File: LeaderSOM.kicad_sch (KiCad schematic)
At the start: 28 parts, among them IC2 TPS1120DR, J1 SWD, J10 SOMConnector, J9 SOMConnector, SW2 Reset, U6 STM32F413RHTx, Y2 8M

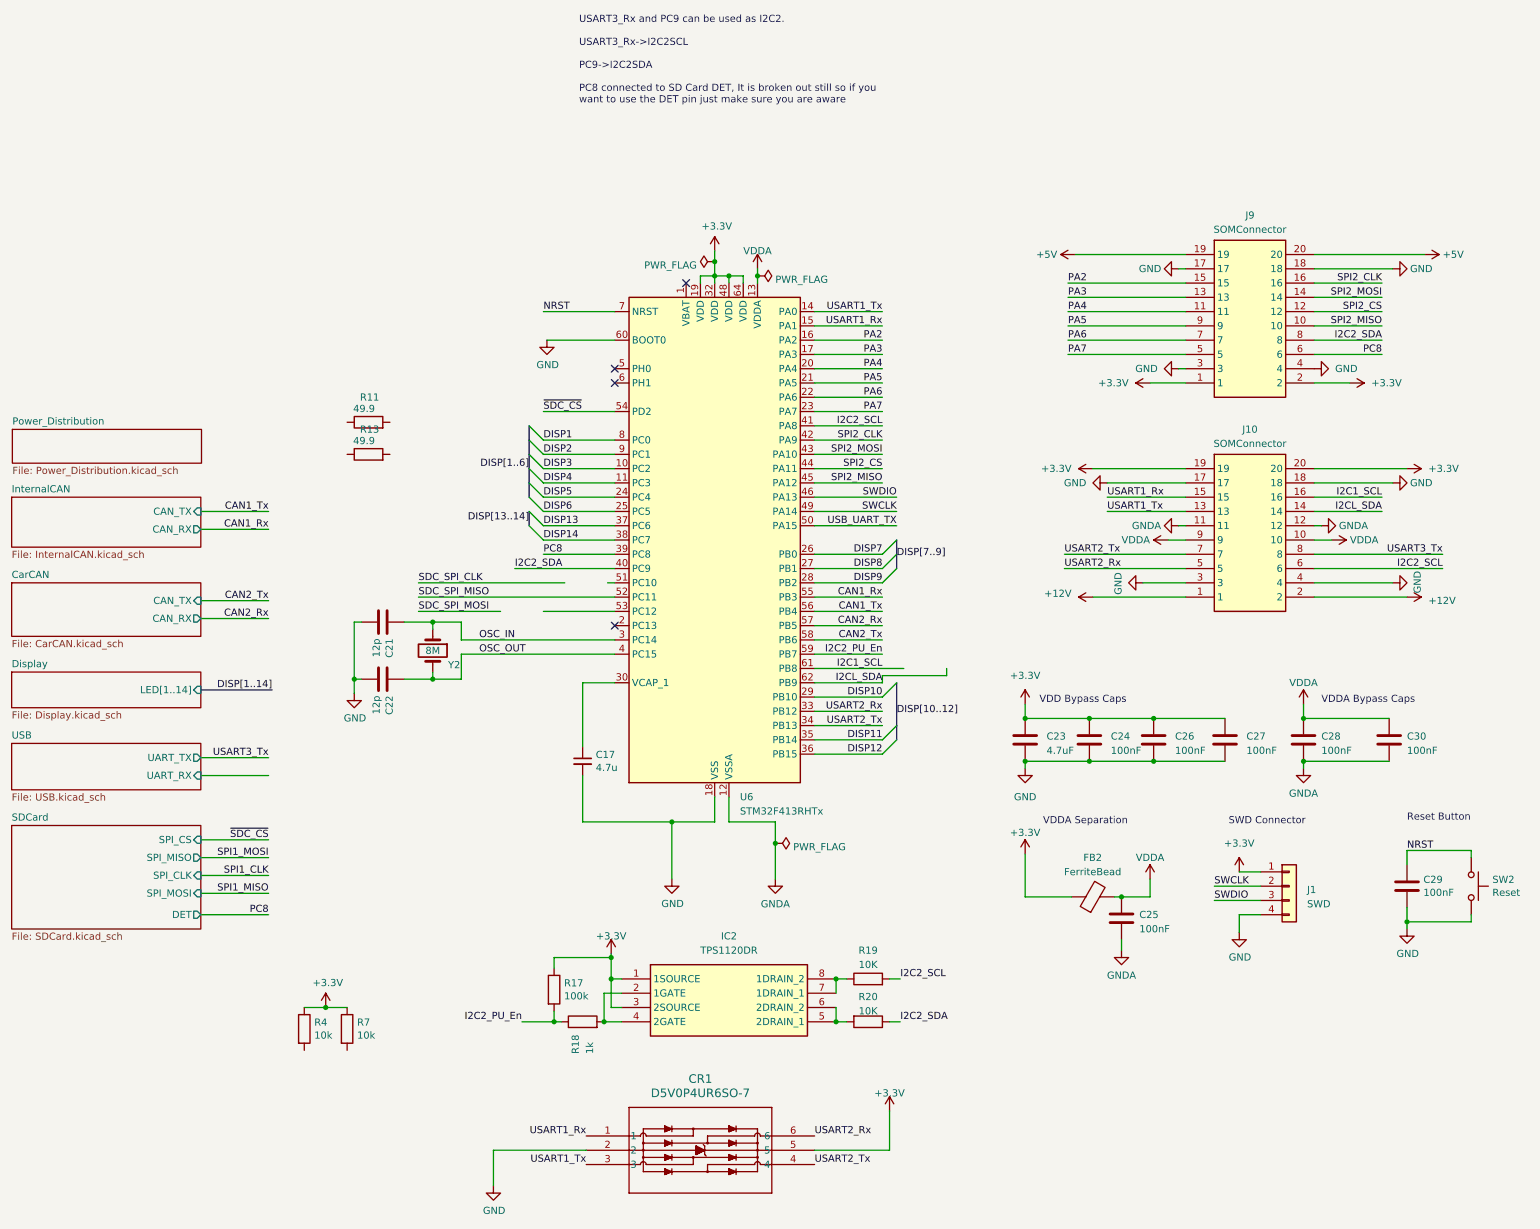
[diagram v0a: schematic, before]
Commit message: updated pin assignments
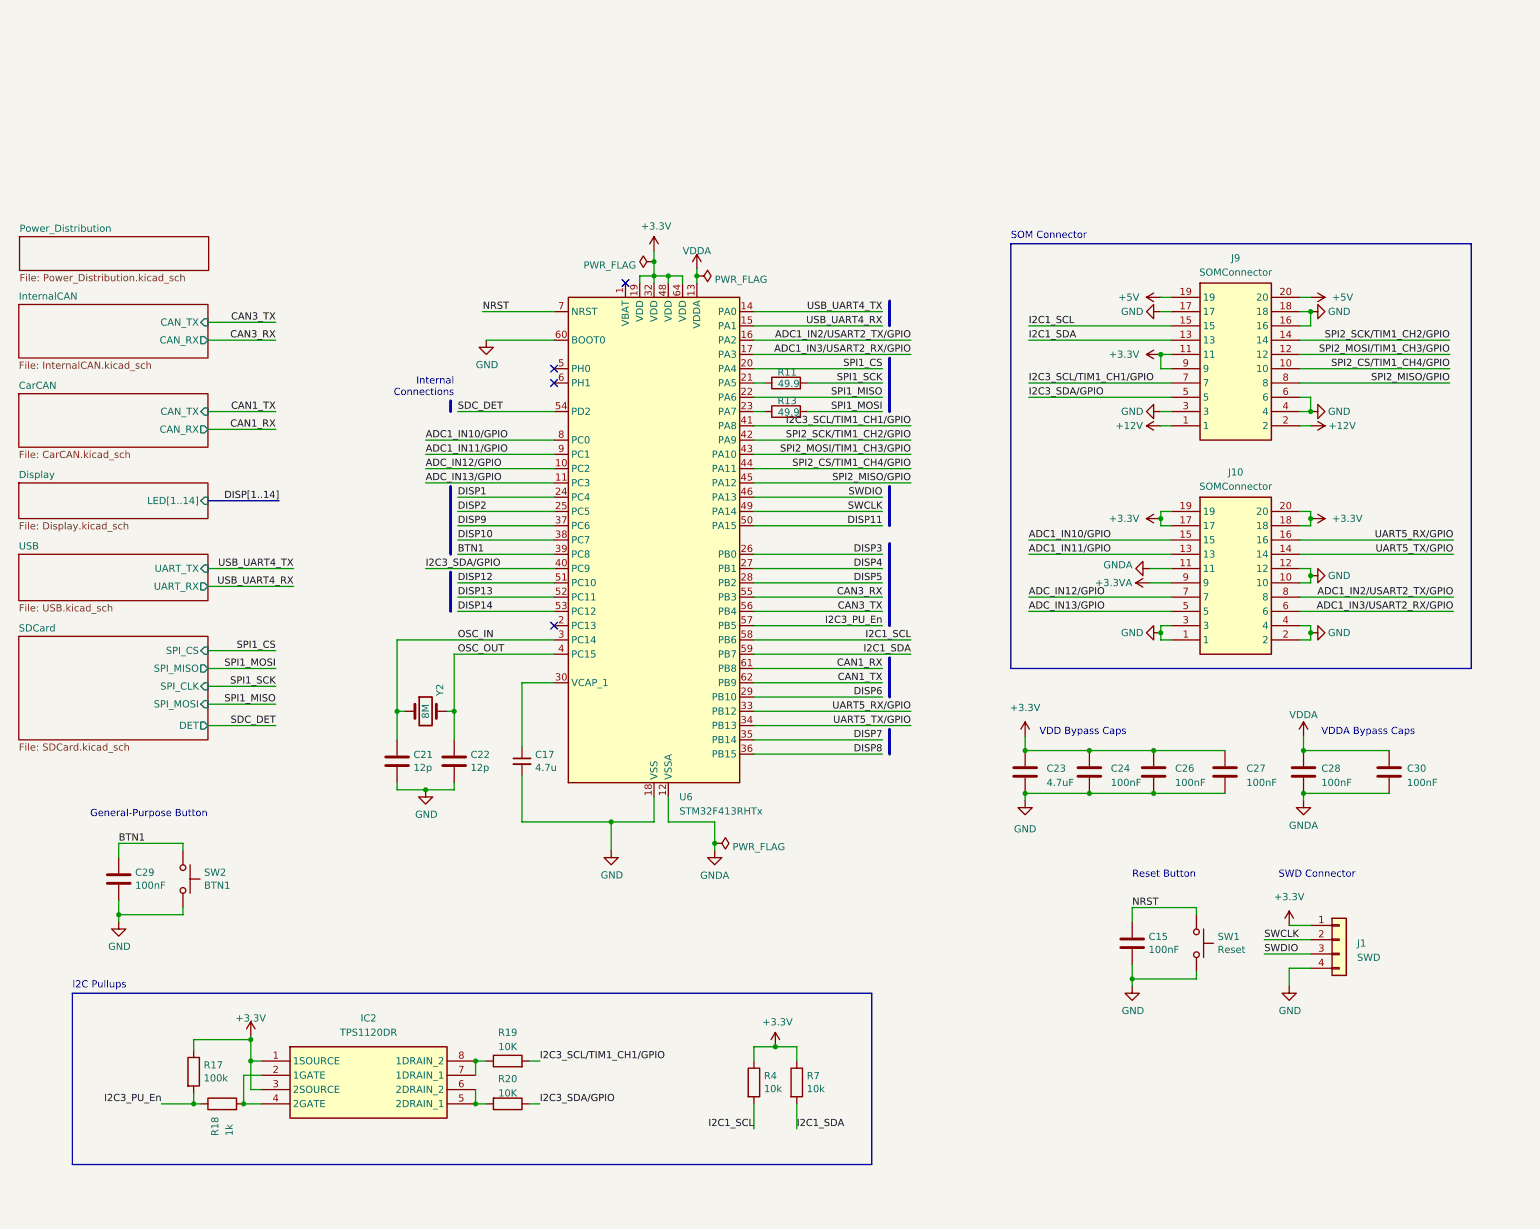
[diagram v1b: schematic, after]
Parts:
- removed C25: 100nF, Capacitor_SMD:C_0805_2012Metric, symbol Device:C
- removed CR1: D5V0P4UR6SO-7, UTSVT_ICs:SOT26_DIO, symbol utsvt-chips:D5V0P4UR6SO-7
- removed FB2: FerriteBead, Inductor_SMD:L_0805_2012Metric, symbol Device:FerriteBead
- added C15: 100nF, Capacitor_SMD:C_0805_2012Metric, symbol Device:C
- added SW1: Reset, Button_Switch_SMD:SW_SPST_B3SL-1002P, symbol Switch:SW_Push
- SW2: value Reset -> BTN1
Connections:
- net CAN2_Tx is gone; now on net I2C1_SCL: U6.58 (PB6)
- net SDC_SPI_MISO is gone; now on net DISP13: U6.52 (PC11)
- net USART3_Tx is gone; now on net ADC1_IN2/USART2_TX/GPIO: J10.8
- net USB_UART_TX is gone; now on net DISP11: U6.50 (PA15)
- net +12V: now also J9.1, J9.2; no longer J10.1, J10.2
- net +3.3V: now also J10.17, J10.18, J9.11, J9.9; no longer J9.1, J9.2
- net DISP1: now also U6.24 (PC4); no longer U6.8 (PC0)
- net DISP10: now also U6.38 (PC7); no longer U6.29 (PB10)
- net DISP11: no longer U6.35 (PB14)
- net DISP12: now also U6.51 (PC10); no longer U6.36 (PB15)
- net DISP13: no longer U6.37 (PC6)
- net DISP14: now also U6.53 (PC12); no longer U6.38 (PC7)
- net DISP2: now also U6.25 (PC5); no longer U6.9 (PC1)
- net DISP3: now also U6.26 (PB0); no longer U6.10 (PC2)
- net DISP4: now also U6.27 (PB1); no longer U6.11 (PC3)
- net DISP5: now also U6.28 (PB2); no longer U6.24 (PC4)
- net DISP6: now also U6.29 (PB10); no longer U6.25 (PC5)
- net DISP7: now also U6.35 (PB14); no longer U6.26 (PB0)
- net DISP8: now also U6.36 (PB15); no longer U6.27 (PB1)
- net DISP9: now also U6.37 (PC6); no longer U6.28 (PB2)
- net GND: now also J10.1, J10.10, J10.12, J10.2, J9.16, J9.6, C15.2, SW1.2; no longer J10.17, J10.18
- net GNDA: no longer J10.12
- net I2C1_SCL: now also J9.15, R4.2; no longer J10.16, U6.61 (PB8)
- net NRST: now also C15.1, SW1.1; no longer C29.1, SW2.1
- net SPI1_MISO: now also U6.22 (PA6)
- net SPI1_MOSI: now also R13.2
- net VDDA: no longer J10.10, J10.9
- net at R13.1: now also U6.23 (PA7)
- net at R11.1: now also U6.21 (PA5)
- net SPI1_SCK: now reaches R11.2
- net I2C1_SDA: now reaches R7.2
- net I2C1_SDA: now also J9.13, U6.59 (PB7)
- net CAN1_Rx renamed CAN3_RX
- net CAN1_Tx renamed CAN3_TX
- net CAN2_Rx renamed I2C3_PU_En
- net I2C3_PU_En: now also R17.2, R18.1
- removed net I2C2_PU_En: R17.2, R18.1, U6.59 (PB7)
- net I2C2_SCL renamed I2C3_SCL/TIM1_CH1/GPIO
- net I2C3_SCL/TIM1_CH1/GPIO: now also J9.7; no longer J10.6
- net I2C2_SDA renamed I2C3_SDA/GPIO
- net I2C3_SDA/GPIO: now also J9.5; no longer J9.8
- net I2CL_SDA renamed CAN1_TX
- net CAN1_TX: no longer J10.14
- net PA2 renamed ADC1_IN2/USART2_TX/GPIO
- net ADC1_IN2/USART2_TX/GPIO: no longer J9.15
- net PA3 renamed ADC1_IN3/USART2_RX/GPIO
- net ADC1_IN3/USART2_RX/GPIO: now also J10.6; no longer J9.13
- net PA4 renamed SPI1_CS
- net SPI1_CS: no longer J9.11
- removed net PA5: J9.9, U6.21 (PA5)
- removed net PA6: J9.7, U6.22 (PA6)
- removed net PA7: J9.5, U6.23 (PA7)
- net PC8 renamed BTN1
- net BTN1: now also C29.1, SW2.1; no longer J9.6
- net SPI2_CLK renamed SPI2_SCK/TIM1_CH2/GPIO
- net SPI2_SCK/TIM1_CH2/GPIO: now also J9.14; no longer J9.16
- net SPI2_CS renamed SPI2_CS/TIM1_CH4/GPIO
- net SPI2_CS/TIM1_CH4/GPIO: now also J9.10; no longer J9.12
- net SPI2_MISO renamed SPI2_MISO/GPIO
- net SPI2_MISO/GPIO: now also J9.8; no longer J9.10
- net SPI2_MOSI renamed SPI2_MOSI/TIM1_CH3/GPIO
- net SPI2_MOSI/TIM1_CH3/GPIO: now also J9.12; no longer J9.14
- net USART1_Rx renamed ADC1_IN10/GPIO
- net ADC1_IN10/GPIO: now also U6.8 (PC0); no longer U6.15 (PA1)
- net USART1_Tx renamed ADC1_IN11/GPIO
- net ADC1_IN11/GPIO: now also U6.9 (PC1); no longer U6.14 (PA0)
- net USART2_Rx renamed ADC_IN13/GPIO
- net ADC_IN13/GPIO: now also U6.11 (PC3); no longer U6.33 (PB12)
- net USART2_Tx renamed ADC_IN12/GPIO
- net ADC_IN12/GPIO: now also U6.10 (PC2); no longer U6.34 (PB13)
- net ~{SDC_CS} renamed SDC_DET
- new net +3.3VA: J10.9
- new net CAN1_RX: U6.61 (PB8)
- new net UART5_RX/GPIO: J10.16, U6.33 (PB12)
- new net UART5_TX/GPIO: J10.14, U6.34 (PB13)
- new net USB_UART4_RX: U6.15 (PA1)
- new net USB_UART4_TX: U6.14 (PA0)
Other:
- note added: "General-Purpose Button"
- note added: "I2C Pullups"
- note added: "Internal Connections"
- note added: "SOM Connector"
- note removed: "USART3_Rx and PC9 can be used as I2C2. USART3_Rx->I2C2SCL PC9->I2C2SDA PC8 connected to SD Card DET, It is broken out still so if you want to use the DET pin just make sure you are aware"
- note removed: "VDDA Separation"
- moved on the sheet: C17, C21, C22, C23, C24, C26, C27, C28, C29, C30, IC2, J1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
